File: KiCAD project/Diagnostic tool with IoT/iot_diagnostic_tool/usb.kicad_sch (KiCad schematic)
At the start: 11 parts

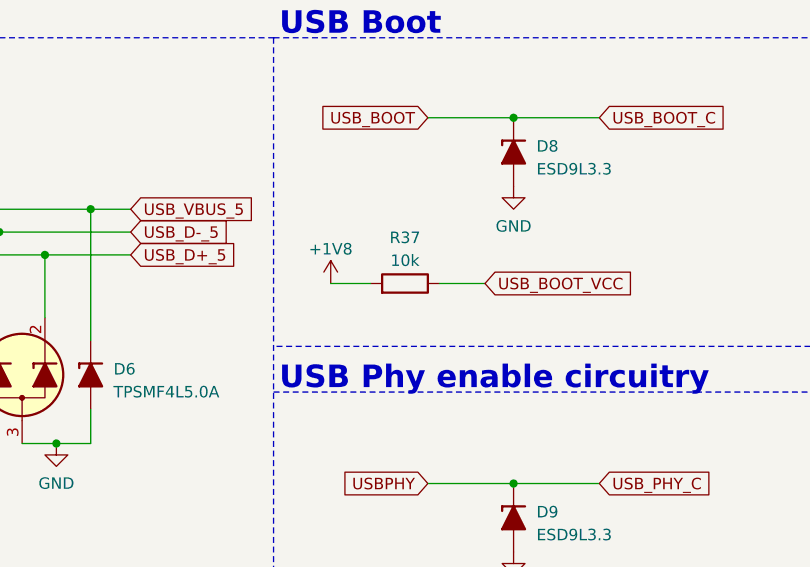
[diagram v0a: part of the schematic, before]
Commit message: Update 17/03/23 - final board update, generated files for manufacturing
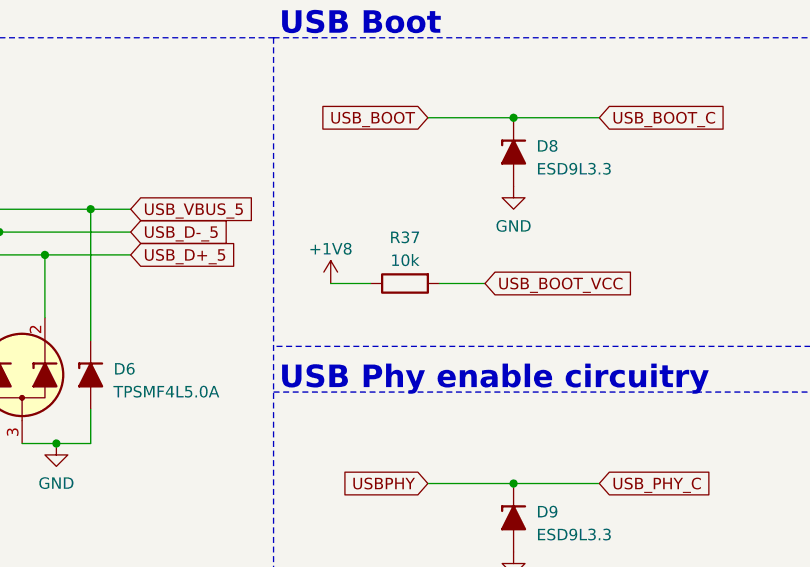
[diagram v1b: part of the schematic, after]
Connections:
- net +1V8: now also R37.1; no longer R37.2
- net USB_BOOT_VCC: now also R37.2; no longer R37.1
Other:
- moved on the sheet: R37
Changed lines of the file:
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@@
     )
   )
-  (symbol (lib_id "Device:R") (at 175.26 99.06 270) (mirror x) (unit 1)
+  (symbol (lib_id "Device:R") (at 175.26 99.06 90) (mirror x) (unit 1)
     (in_bom yes) (on_board yes) (dnp no) (fields_autoplaced)
     (property "Reference" "R37" (at 175.26 93.98 90)
@@
       (effects (font (size 1.27 1.27)))
     )
-    (property "Footprint" "Resistor_SMD:R_0402_1005Metric" (at 175.26 100.838 90)
+    (property "Footprint" "Resistor_SMD:R_0402_1005Metric" (at 175.26 97.282 90)
       (effects (font (size 1.27 1.27)) hide)
     )
